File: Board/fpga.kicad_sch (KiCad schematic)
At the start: 16 parts, among them U1 XC6SLX9-TQG144

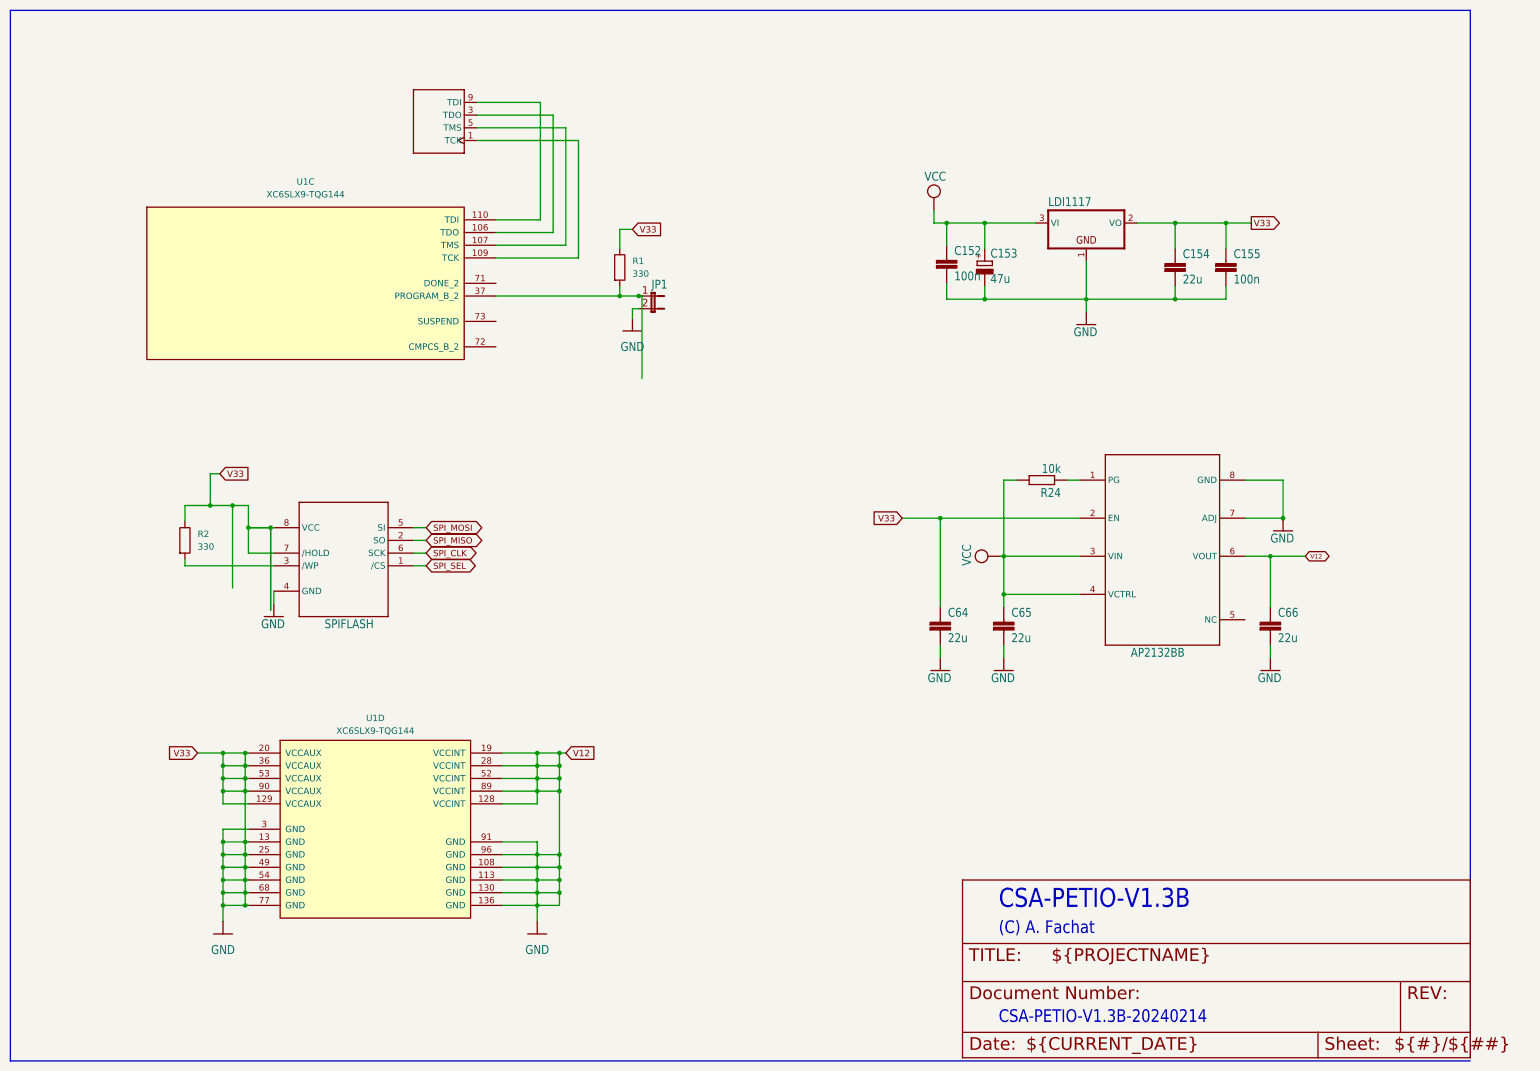
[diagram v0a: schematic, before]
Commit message: update
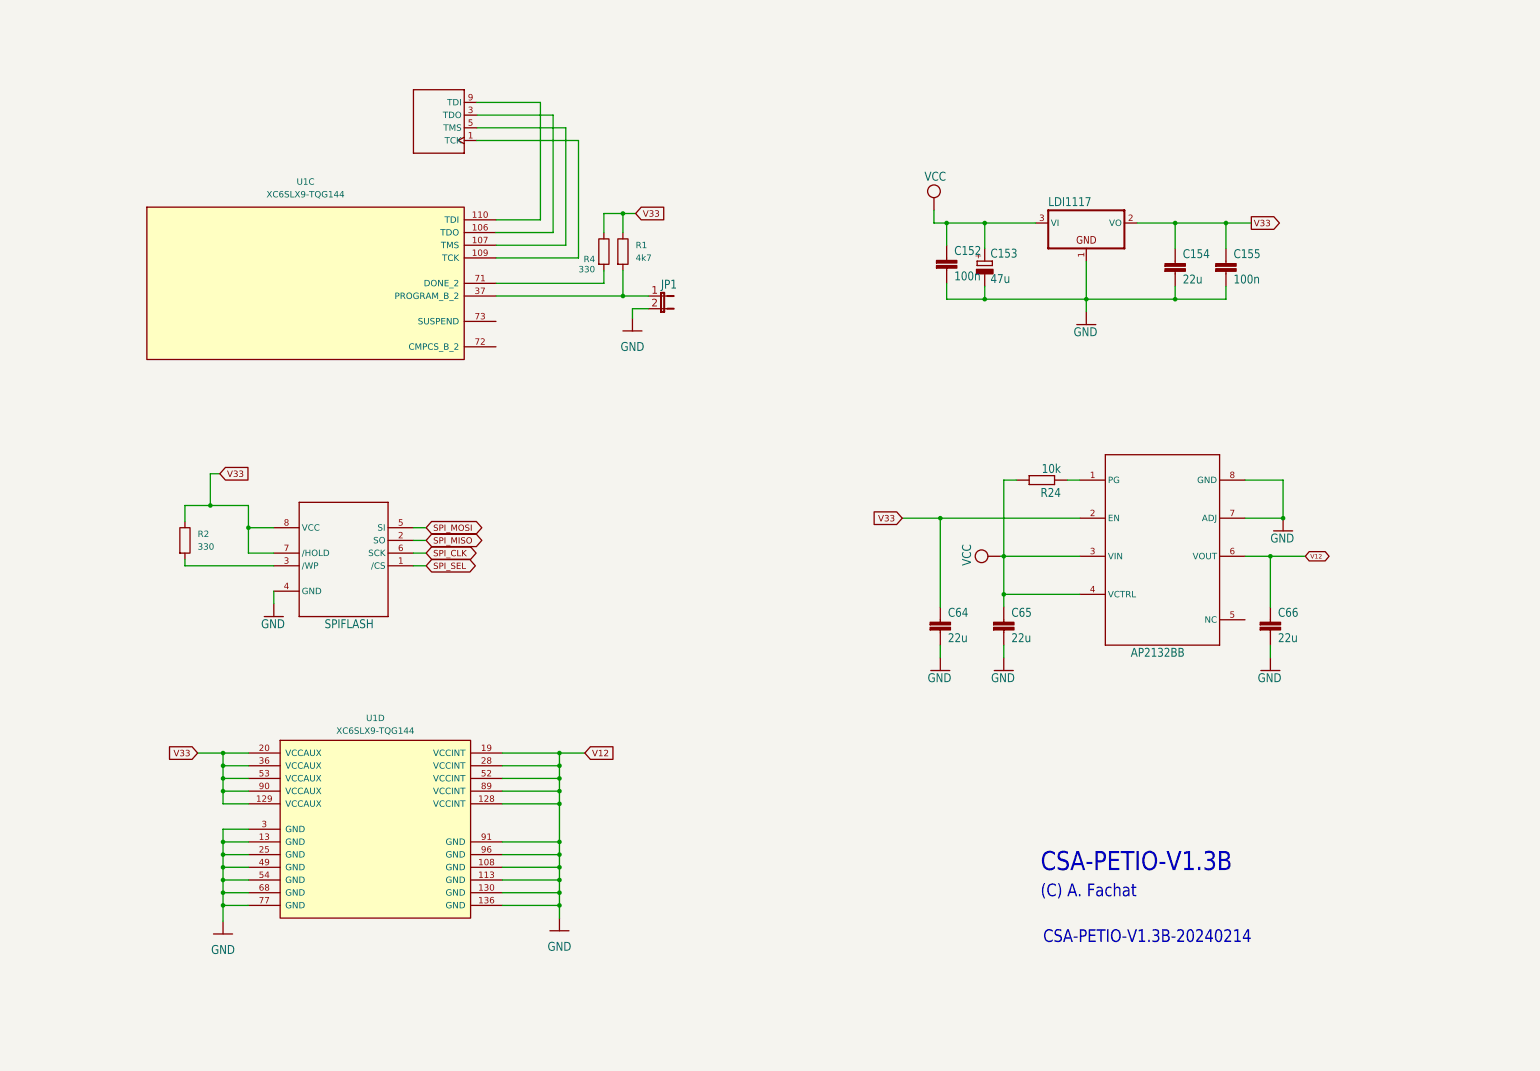
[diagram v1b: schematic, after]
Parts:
- added R4: 330, Resistor_SMD:R_0603_1608Metric_Pad0.98x0.95mm_HandSolder, symbol Device:R
- R1: value 330 -> 4k7
- UX16: footprint cbm_ultipet_v1:PSOP-8-FIXED -> Package_SO:Diodes_PSOP-8
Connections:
- net GND: no longer C154.1, C155.1, C64.1, R1.1, R2.1, U1.129 (VCCAUX), U1.20 (VCCAUX), U1.36 (VCCAUX), U1.53 (VCCAUX), U1.90 (VCCAUX), UX16.2 (EN), UX17.2 (VO), UX18.7 (/HOLD), UX18.8 (VCC)
- net at U1.71 (DONE_2): now also R4.2
- new net V33: C154.1, C155.1, C64.1, R1.1, R2.1, R4.1, U1.129 (VCCAUX), U1.20 (VCCAUX), U1.36 (VCCAUX), U1.53 (VCCAUX), U1.90 (VCCAUX), UX16.2 (EN), UX17.2 (VO), UX18.7 (/HOLD), UX18.8 (VCC)
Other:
- moved on the sheet: JP1, R1
